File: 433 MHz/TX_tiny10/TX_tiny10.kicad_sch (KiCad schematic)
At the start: 8 parts, among them J1 Conn_01x03, J2 AVR-ISP-6, U1 ATtiny10-TS

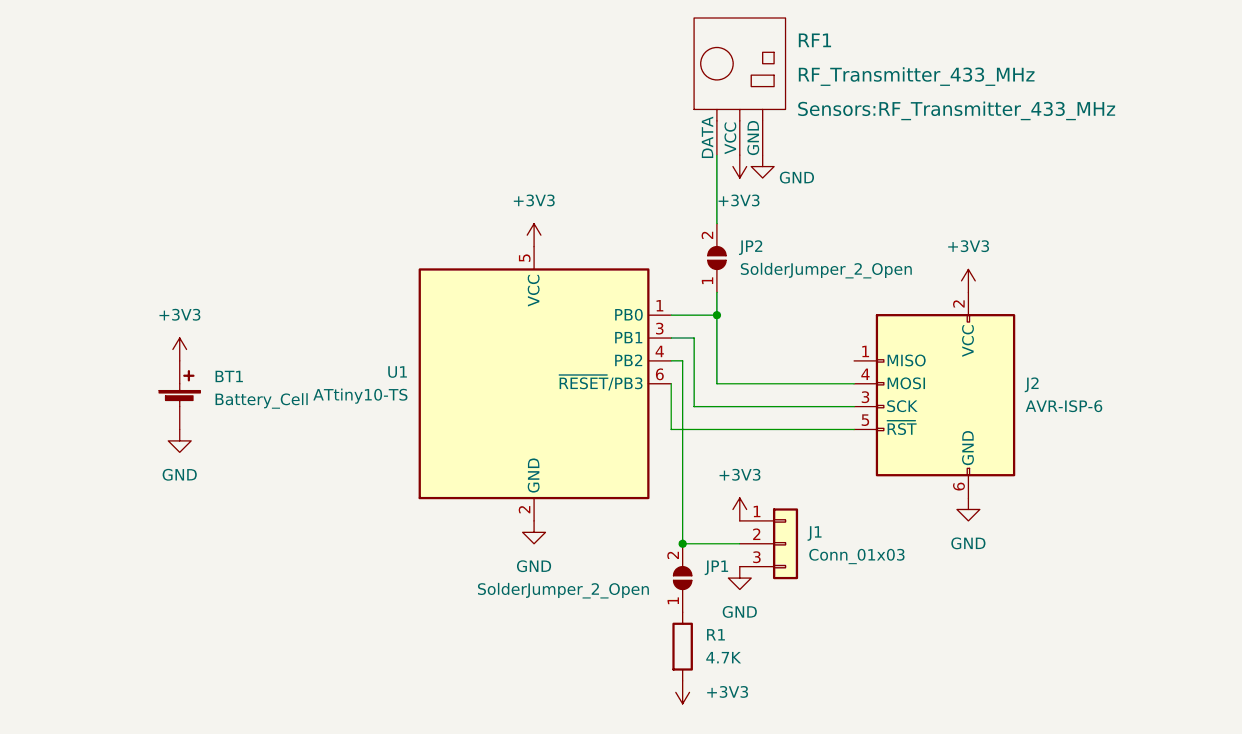
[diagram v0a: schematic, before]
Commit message: 01.07.2022
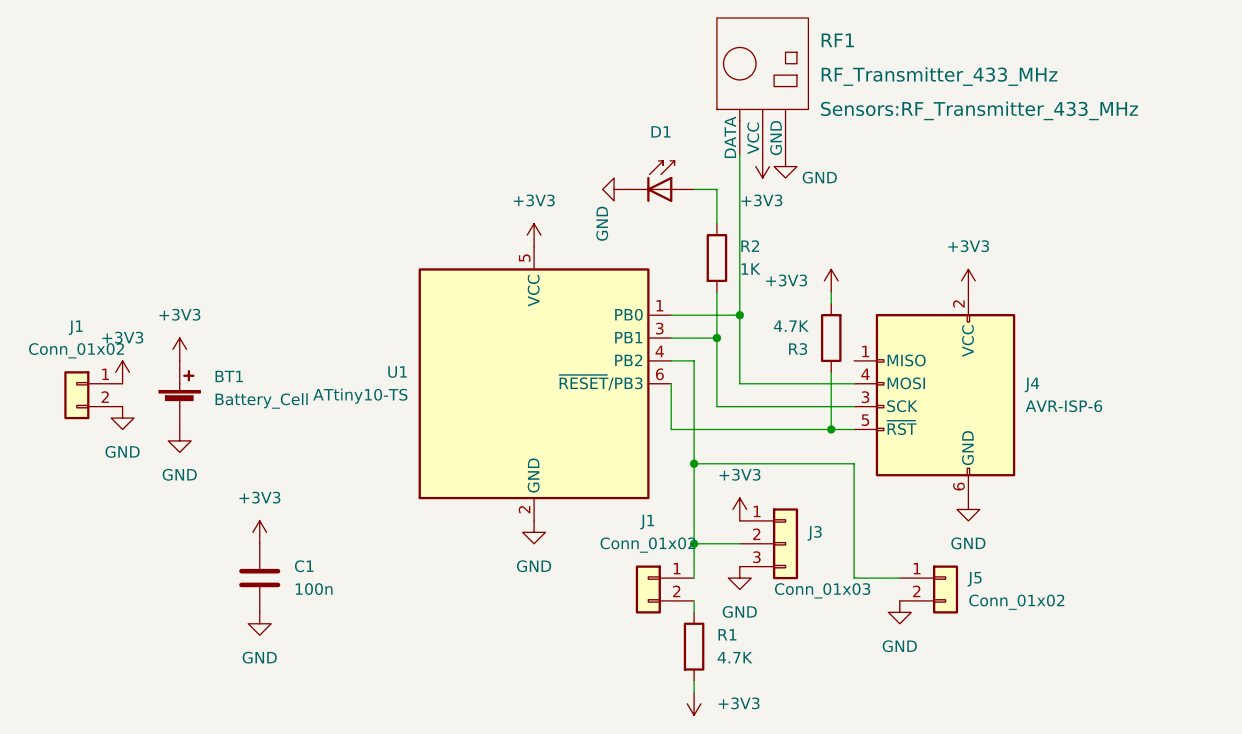
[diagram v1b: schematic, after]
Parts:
- removed JP1, JP2: SolderJumper_2_Open, Jumper:SolderJumper-2_P1.3mm_Open_TrianglePad1.0x1.5mm, symbol Jumper:SolderJumper_2_Open
- added C1: 100n, Capacitor_SMD:C_0805_2012Metric, symbol Device:C
- added D1: SFH4346, LED_THT:LED_D3.0mm, symbol LED:SFH4346
- added J1 (x2), J5: Conn_01x02, Connector_PinHeader_2.54mm:PinHeader_1x02_P2.54mm_Vertical, symbol Connector_Generic:Conn_01x02
- added R2, R3: 4.7K, Resistor_SMD:R_0805_2012Metric, symbol Device:R
- renumbered J1 to J3, J2 to J4
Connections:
- net +3V3: now also C1.1, J1.1 (Pin_1), R3.2
- net GND: now also C1.2, D1.1 (K), J1.2 (Pin_2), J5.2 (Pin_2)
- net at R1.1: now also J1.2 (Pin_2)
- net at J3.2 (Pin_2), U1.4 (PB2): now also J1.1 (Pin_1), J5.1 (Pin_1)
- net at J4.4 (MOSI), U1.1 (PB0): now also RF1.1 (DATA)
- net at J4.3 (SCK), U1.3 (PB1): now also R2.2
- net at J4.5 (~{RST}), U1.6 (~{RESET}/PB3): now also R3.1
- new net: D1.2 (A), R2.1
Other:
- moved on the sheet: R1, RF1
